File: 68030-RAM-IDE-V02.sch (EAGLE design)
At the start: 73 parts, among them IC1 REG1117, IC10 ICS570B, IC2 74HCT245PW, IC3 74AC16245, IC4 AM29F010S, IC5 74ALVT16543, IC6 74ALVT16543, IC7 XC95288XL-TQ144, IC8 K4S56163, IC9 K4S56163, J1 22-05-7028-02, X1 MABC96R

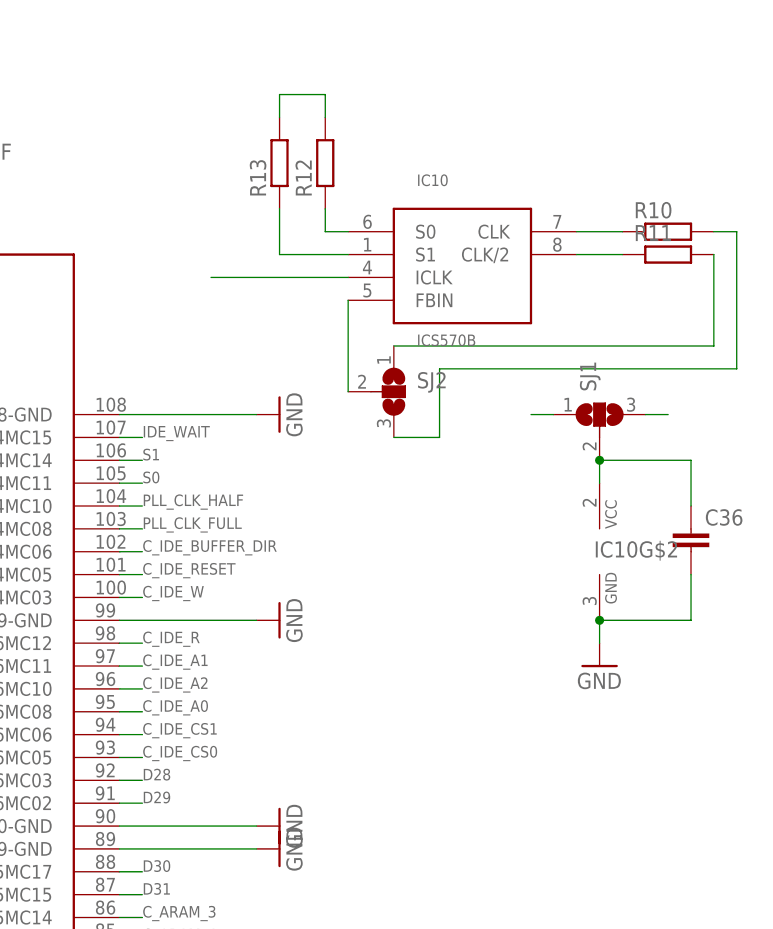
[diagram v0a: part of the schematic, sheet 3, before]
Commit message: fooling around mit cl2
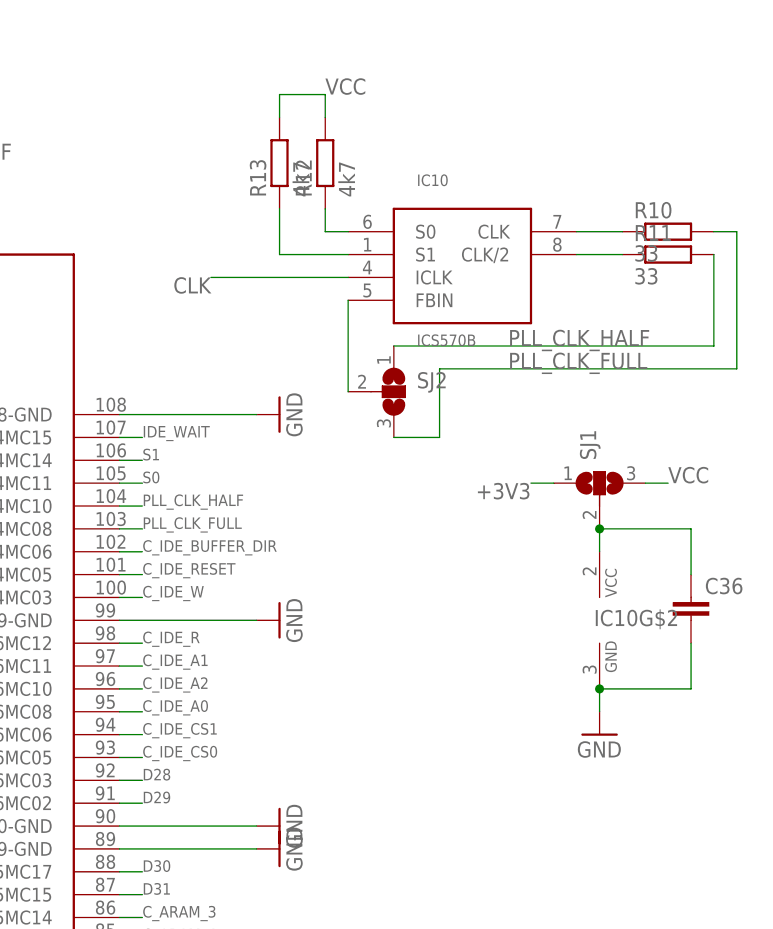
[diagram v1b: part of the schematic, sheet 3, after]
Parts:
- R10, R11: value (none) -> 33
- R12, R13: value (none) -> 4k7
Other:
- moved on the sheet: C36, IC10G$2, SJ1
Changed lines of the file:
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@@
 <part name="SJ1" library="jumper" deviceset="SJ2W" device=""/>
 <part name="C36" library="rcl" deviceset="C-EU" device="C0603K"/>
-<part name="R10" library="rcl" deviceset="R-EU_" device="R0603"/>
-<part name="R11" library="rcl" deviceset="R-EU_" device="R0603"/>
-<part name="R12" library="rcl" deviceset="R-EU_" device="R0603"/>
-<part name="R13" library="rcl" deviceset="R-EU_" device="R0603"/>
+<part name="R10" library="rcl" deviceset="R-EU_" device="R0603" value="33"/>
+<part name="R11" library="rcl" deviceset="R-EU_" device="R0603" value="33"/>
+<part name="R12" library="rcl" deviceset="R-EU_" device="R0603" value="4k7"/>
+<part name="R13" library="rcl" deviceset="R-EU_" device="R0603" value="4k7"/>
 <part name="SJ2" library="jumper" deviceset="SJ2W" device=""/>
 <part name="C37" library="rcl" deviceset="C-EU" device="C0603K" value="100pF"/>
@@
 <instance part="GND33" gate="1" x="66.04" y="5.08"/>
 <instance part="IC10" gate="G$1" x="200.66" y="142.24"/>
-<instance part="IC10" gate="G$2" x="215.9" y="116.84"/>
-<instance part="GND34" gate="1" x="215.9" y="104.14"/>
-<instance part="SJ1" gate="G$1" x="215.9" y="132.08" rot="R90"/>
-<instance part="C36" gate="G$1" x="226.06" y="119.38"/>
+<instance part="IC10" gate="G$2" x="215.9" y="109.22"/>
+<instance part="GND34" gate="1" x="215.9" y="96.52"/>
+<instance part="SJ1" gate="G$1" x="215.9" y="124.46" rot="R90"/>
+<instance part="C36" gate="G$1" x="226.06" y="111.76"/>
 <instance part="R10" gate="G$1" x="223.52" y="152.4"/>
 <instance part="R11" gate="G$1" x="223.52" y="149.86"/>
@@
 <pinref part="GND34" gate="1" pin="GND"/>
 <pinref part="IC10" gate="G$2" pin="GND"/>
-<wire x1="215.9" y1="106.68" x2="215.9" y2="109.22" width="0.1524" layer="91"/>
+<wire x1="215.9" y1="99.06" x2="215.9" y2="101.6" width="0.1524" layer="91"/>
 <pinref part="C36" gate="G$1" pin="2"/>
-<wire x1="215.9" y1="109.22" x2="226.06" y2="109.22" width="0.1524" layer="91"/>
-<wire x1="226.06" y1="109.22" x2="226.06" y2="114.3" width="0.1524" layer="91"/>
-<junction x="215.9" y="109.22"/>
+<wire x1="215.9" y1="101.6" x2="226.06" y2="101.6" width="0.1524" layer="91"/>
+<wire x1="226.06" y1="101.6" x2="226.06" y2="106.68" width="0.1524" layer="91"/>
+<junction x="215.9" y="101.6"/>
 </segment>
 <segment>
@@
 <segment>
 <pinref part="SJ1" gate="G$1" pin="1"/>
-<wire x1="210.82" y1="132.08" x2="208.28" y2="132.08" width="0.1524" layer="91"/>
+<wire x1="210.82" y1="124.46" x2="208.28" y2="124.46" width="0.1524" layer="91"/>
+<label x="208.28" y="124.46" size="1.778" layer="95" rot="R180"/>
 </segment>
 </net>
@@
 <pinref part="IC10" gate="G$1" pin="ICLK"/>
 <wire x1="187.96" y1="147.32" x2="172.72" y2="147.32" width="0.1524" layer="91"/>
+<label x="172.72" y="147.32" size="1.778" layer="95" rot="R180"/>
 </segment>
 </net>
@@
 <segment>
 <pinref part="C36" gate="G$1" pin="1"/>
-<wire x1="226.06" y1="121.92" x2="226.06" y2="127" width="0.1524" layer="91"/>
+<wire x1="226.06" y1="114.3" x2="226.06" y2="119.38" width="0.1524" layer="91"/>
 <pinref part="SJ1" gate="G$1" pin="2"/>
-<wire x1="226.06" y1="127" x2="215.9" y2="127" width="0.1524" layer="91"/>
+<wire x1="226.06" y1="119.38" x2="215.9" y2="119.38" width="0.1524" layer="91"/>
 <pinref part="IC10" gate="G$2" pin="VCC"/>
-<wire x1="215.9" y1="127" x2="215.9" y2="124.46" width="0.1524" layer="91"/>
-<junction x="215.9" y="127"/>
+<wire x1="215.9" y1="119.38" x2="215.9" y2="116.84" width="0.1524" layer="91"/>
+<junction x="215.9" y="119.38"/>
 </segment>
 </net>
@@
 <segment>
 <pinref part="SJ1" gate="G$1" pin="3"/>
-<wire x1="220.98" y1="132.08" x2="223.52" y2="132.08" width="0.1524" layer="91"/>
+<wire x1="220.98" y1="124.46" x2="223.52" y2="124.46" width="0.1524" layer="91"/>
+<label x="223.52" y="124.46" size="1.778" layer="95"/>
 </segment>
 <segment>
@@
 <pinref part="R12" gate="G$1" pin="2"/>
 <wire x1="185.42" y1="167.64" x2="185.42" y2="165.1" width="0.1524" layer="91"/>
+<label x="185.42" y="167.64" size="1.778" layer="95"/>
 </segment>
 </net>
@@
 <pinref part="SJ2" gate="G$1" pin="3"/>
 <wire x1="198.12" y1="129.54" x2="193.04" y2="129.54" width="0.1524" layer="91"/>
+<label x="205.74" y="137.16" size="1.778" layer="95"/>
 </segment>
 <segment>
@@
 <pinref part="SJ2" gate="G$1" pin="1"/>
 <wire x1="228.6" y1="139.7" x2="193.04" y2="139.7" width="0.1524" layer="91"/>
+<label x="205.74" y="139.7" size="1.778" layer="95"/>
 </segment>
 <segment>
